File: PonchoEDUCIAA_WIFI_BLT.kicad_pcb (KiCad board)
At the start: 2 copper layers, 25 parts, among them J1 UART, SW1 Reset, SW2 Boot, U1 ESP32-WROOM

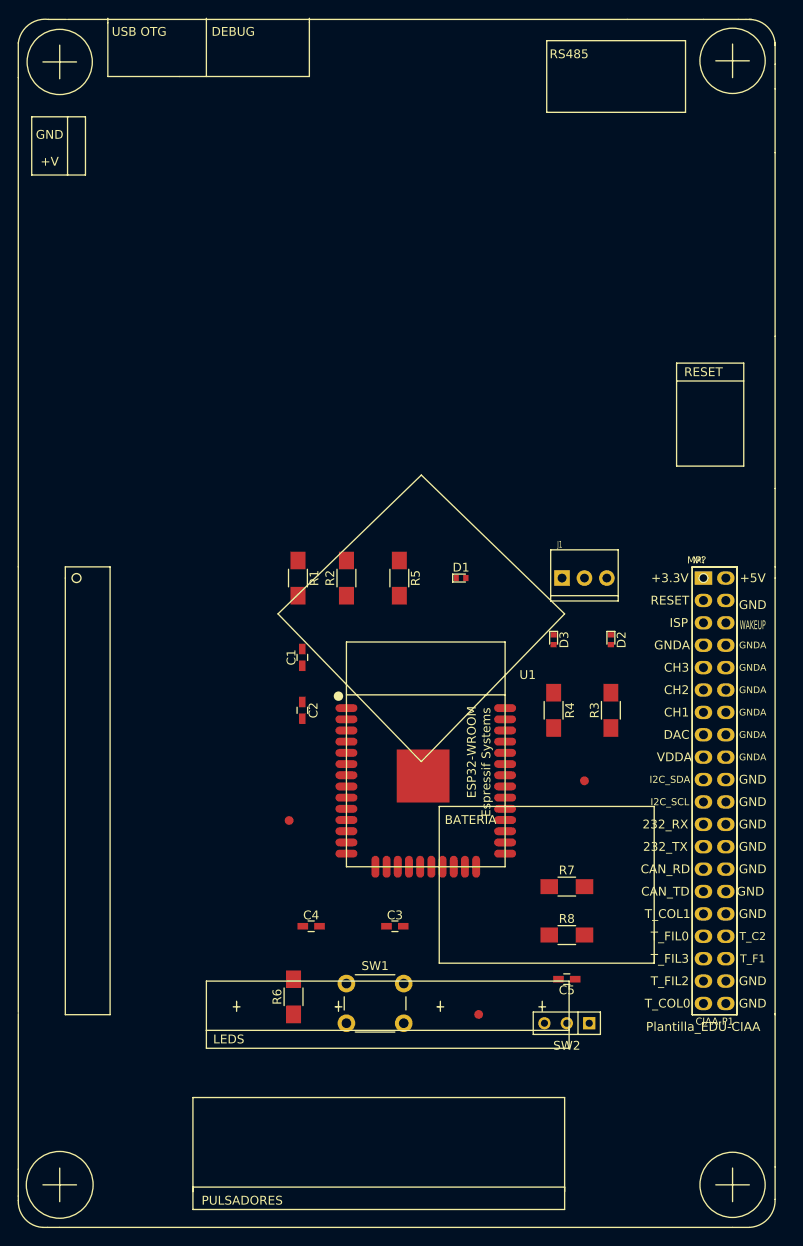
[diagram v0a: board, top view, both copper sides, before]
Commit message: Revision del proyecto
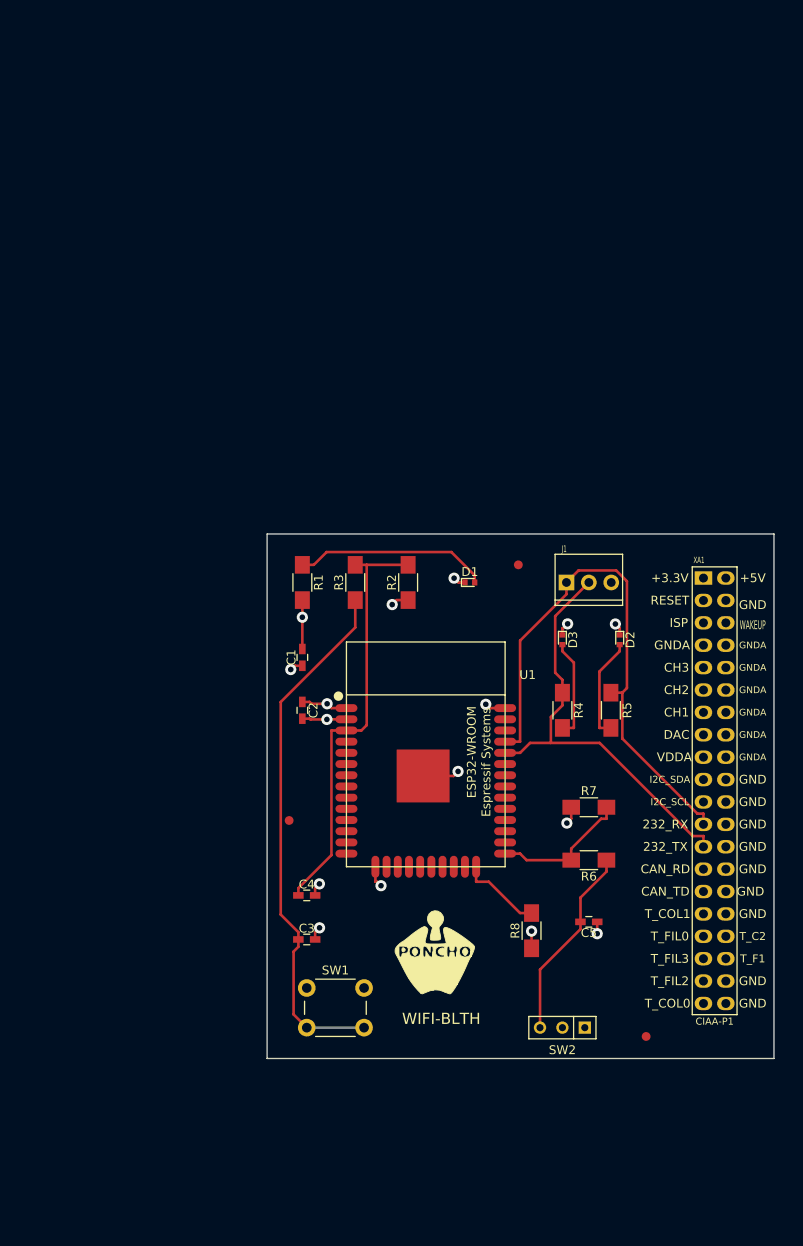
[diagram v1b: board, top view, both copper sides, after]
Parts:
- removed MP?: Plantilla_EDU-CIAA, PonchoEDUCIAA_WIFI_BLTH:Plantilla_EDU-CIAA
- added G1: WIFI-BLTH, PonchoEDUCIAA_WIFI_BLTH:Logo_Poncho, F.Cu at (148.0, 121.5)
- R1, R4, R5: value 400 -> 402
- moved R6 36.9 mm to (165.5, 111.0), turned to 180 degrees
- moved R3 32.4 mm to (139.0, 79.5)
- moved R5 28.3 mm to (168.0, 94.0)
- moved F3 25.6 mm to (157.5, 77.5)
- moved F1 19.2 mm to (172.0, 131.0)
- moved C3 10.1 mm to (133.5, 120.0)
- moved R7 9.34 mm to (165.5, 105.0)
- moved R2 7.02 mm to (145.0, 79.5)
- moved C5 6.96 mm to (165.5, 118.0)
- moved SW1 4.53 mm to (133.5, 125.5)
- moved R8 4.03 mm to (159.0, 119.0), turned to 90 degrees
- moved C4 3.54 mm to (133.5, 115.0)
- moved D1 1.12 mm to (152.0, 79.5)
- moved D2 1.00 mm to (169.0, 86.0)
- moved D3 1.00 mm to (162.5, 86.0)
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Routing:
- net Net-(J1-Pad1): track 0.00 -> 63.2 mm
- net Net-(C3-Pad1): track 0.00 -> 60.2 mm
- net Net-(J1-Pad2): track 0.00 -> 49.2 mm
- net Net-(C4-Pad1): track 0.00 -> 48.7 mm
- net GND: track 0.00 -> 26.6 mm, vias 0 -> 12
- net Net-(C5-Pad2): track 0.00 -> 22.1 mm
- net Net-(D1-Pad2): track 0.00 -> 22.0 mm
- net Net-(R6-Pad2): track 0.00 -> 15.8 mm
- net +3V3: track 0.00 -> 14.6 mm, vias 0 -> 4
- net Net-(D2-Pad2): track 0.00 -> 11.7 mm
- net Net-(D3-Pad2): track 0.00 -> 11.3 mm
- net Net-(R8-Pad2): track 0.00 -> 9.46 mm
- added copper zone on Power, net +3V3
- added copper zone on GND, net GND
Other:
- board outline added: 57.5 x 59.5 mm
- copper layers 2 -> 4
